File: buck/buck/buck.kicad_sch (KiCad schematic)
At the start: 34 parts, among them M1 CSD19537Q3, M2 CSD19537Q3, U1 LM5146RGYR

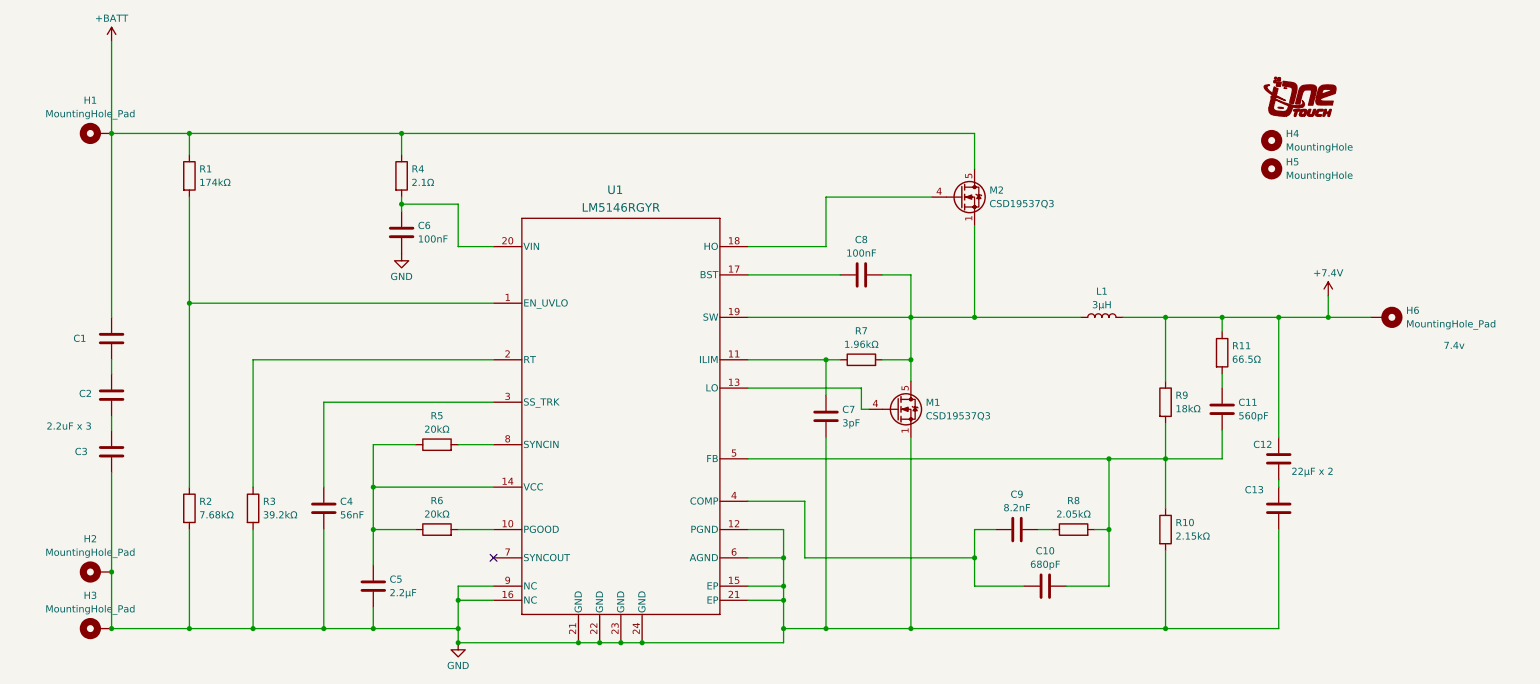
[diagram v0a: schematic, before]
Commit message: PCB updates
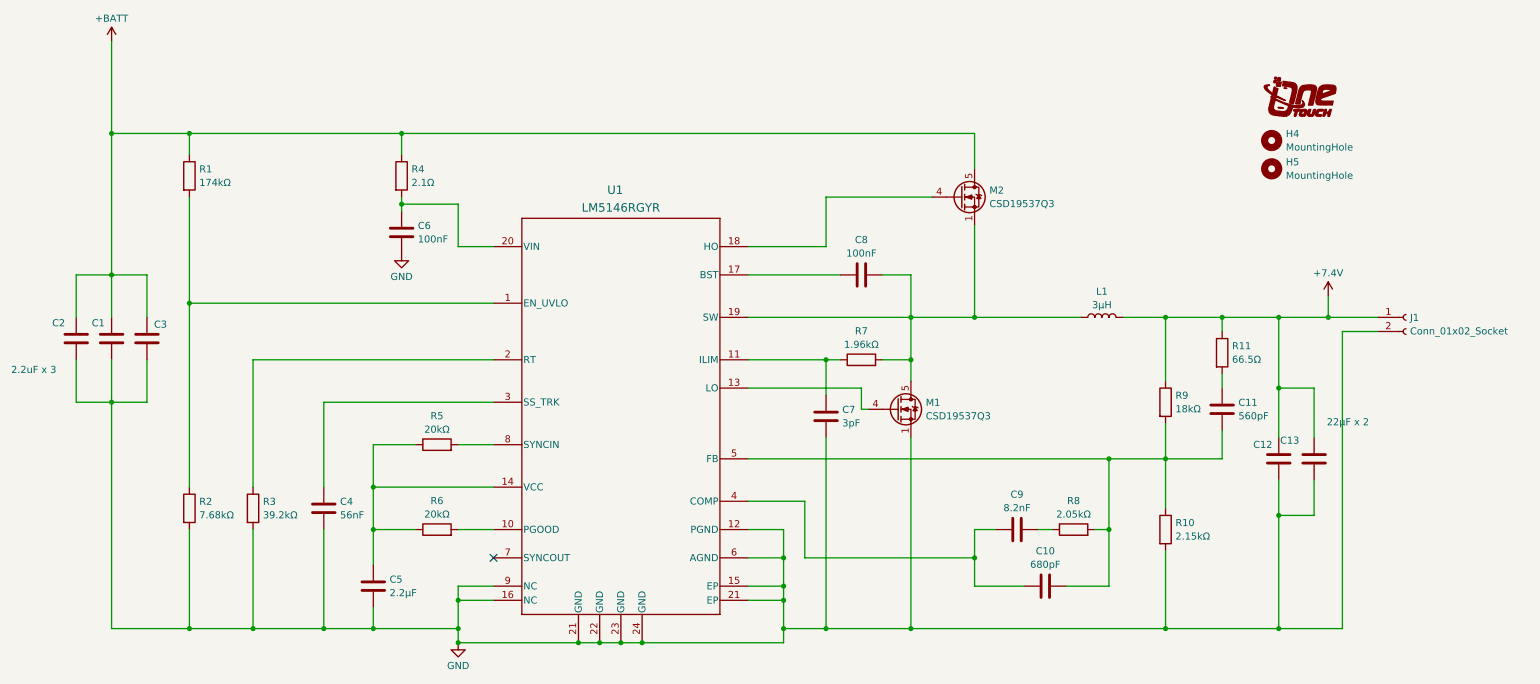
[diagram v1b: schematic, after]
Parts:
- removed H1, H2, H3, H6: MountingHole_Pad, TestPoint:TestPoint_Pad_4.0x7.4mm, symbol Mechanical:MountingHole_Pad
- added J1: Conn_01x02_Socket, Connector_JST:JST_XH_S2B-XH-A_1x02_P2.50mm_Horizontal, symbol Connector:Conn_01x02_Socket
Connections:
- net +7.4V: now also C13.1, J1.1 (Pin_1)
- net +BATT: now also C2.1, C3.1
- net GND: now also C1.2, C12.2, C2.2, J1.2 (Pin_2)
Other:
- moved on the sheet: C13, C2, C3
